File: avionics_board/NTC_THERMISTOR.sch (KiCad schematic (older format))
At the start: 2 parts

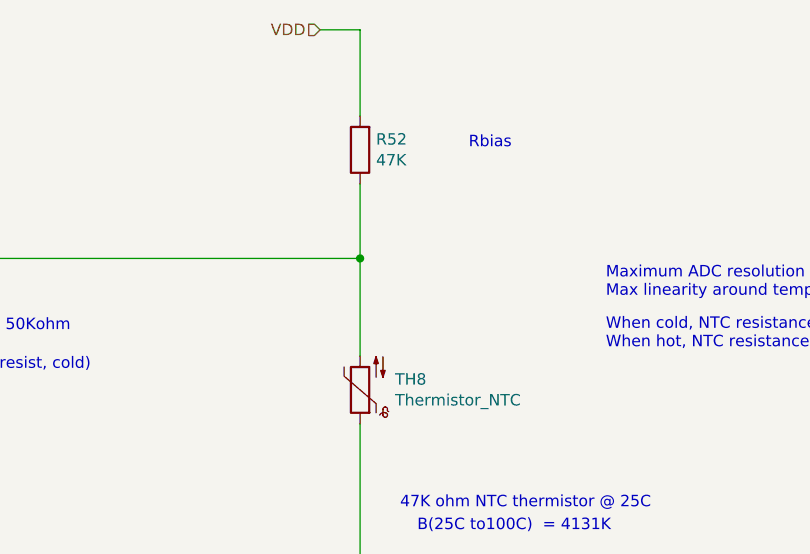
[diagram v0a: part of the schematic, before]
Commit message: Progress on EPS
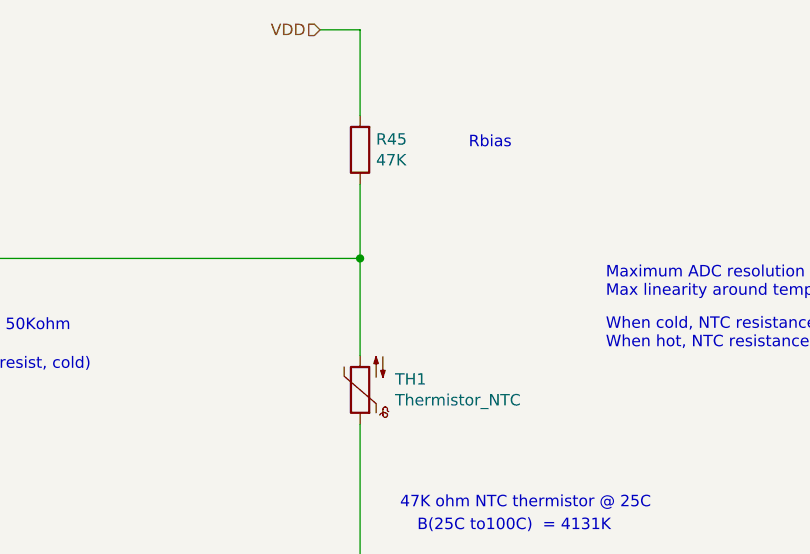
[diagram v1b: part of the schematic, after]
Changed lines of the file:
@@
 $Descr A 11000 8500
 encoding utf-8
-Sheet 14 25
+Sheet 13 24
 Title "NTC THERMISTOR"
 Date "2020-05-05"
@@
 AR Path="/5EA31C93/5EAB0B79/5EC02E3E/5EB42947" Ref="R51"  Part="1"
 AR Path="/5EA31C93/5EAB0B79/5EC02E43/5EB42947" Ref="R52"  Part="1"
-F 0 "R52" H 4680 1854 50  0000 R CNN
+F 0 "R45" H 4680 1854 50  0000 R CNN
 F 1 "47K" H 4680 1945 50  0000 R CNN
 F 2 "Resistor_SMD:R_0603_1608Metric_Pad1.05x0.95mm_HandSolder" V 4680 1900 50  0001 C CNN
@@
 AR Path="/5EA31C93/5EAB0B79/5EC02E3E/5EB41DDD" Ref="TH7"  Part="1"
 AR Path="/5EA31C93/5EAB0B79/5EC02E43/5EB41DDD" Ref="TH8"  Part="1"
-F 0 "TH8" H 4597 2904 50  0000 R CNN
+F 0 "TH1" H 4597 2904 50  0000 R CNN
 F 1 "Thermistor_NTC" H 4597 2995 50  0000 R CNN
 F 2 "Connector_PinHeader_1.27mm:PinHeader_1x02_P1.27mm_Vertical" H 4750 3000 50  0001 C CNN

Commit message: Essentially done with EPS schematic
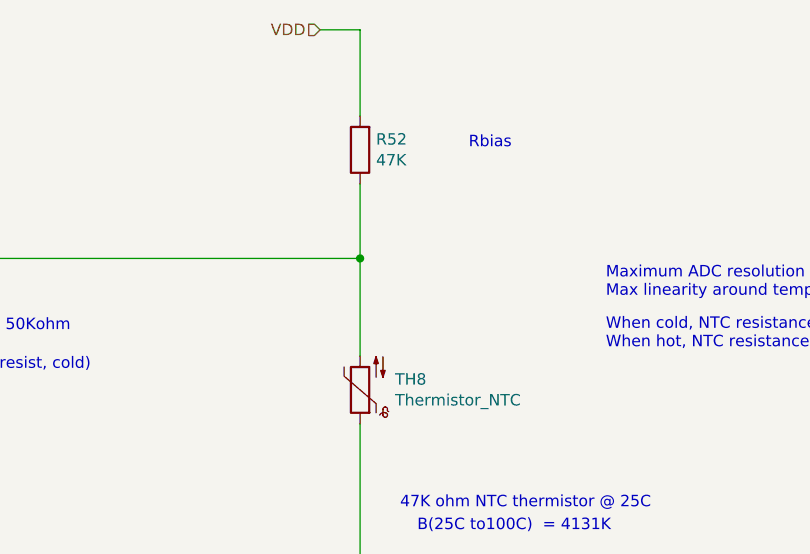
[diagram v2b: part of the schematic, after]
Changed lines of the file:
@@
 $Descr A 11000 8500
 encoding utf-8
-Sheet 13 24
+Sheet 13 23
 Title "NTC THERMISTOR"
 Date "2020-05-05"
@@
 AR Path="/5EA31C93/5EAB0B79/5EC02E3E/5EB42947" Ref="R51"  Part="1"
 AR Path="/5EA31C93/5EAB0B79/5EC02E43/5EB42947" Ref="R52"  Part="1"
-F 0 "R45" H 4680 1854 50  0000 R CNN
+F 0 "R52" H 4680 1854 50  0000 R CNN
 F 1 "47K" H 4680 1945 50  0000 R CNN
 F 2 "Resistor_SMD:R_0603_1608Metric_Pad1.05x0.95mm_HandSolder" V 4680 1900 50  0001 C CNN
@@
 AR Path="/5EA31C93/5EAB0B79/5EC02E3E/5EB41DDD" Ref="TH7"  Part="1"
 AR Path="/5EA31C93/5EAB0B79/5EC02E43/5EB41DDD" Ref="TH8"  Part="1"
-F 0 "TH1" H 4597 2904 50  0000 R CNN
+F 0 "TH8" H 4597 2904 50  0000 R CNN
 F 1 "Thermistor_NTC" H 4597 2995 50  0000 R CNN
 F 2 "Connector_PinHeader_1.27mm:PinHeader_1x02_P1.27mm_Vertical" H 4750 3000 50  0001 C CNN

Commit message: Update Avionics part names to match KiCad update. Update Avionics board to use new interboard connector
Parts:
- R45: footprint Resistor_SMD:R_0603_1608Metric_Pad1.05x0.95mm_HandSolder -> Resistor_SMD:R_0603_1608Metric_Pad0.98x0.95mm_HandSolder
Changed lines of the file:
@@
 F 0 "R52" H 4680 1854 50  0000 R CNN
 F 1 "47K" H 4680 1945 50  0000 R CNN
-F 2 "Resistor_SMD:R_0603_1608Metric_Pad1.05x0.95mm_HandSolder" V 4680 1900 50  0001 C CNN
+F 2 "Resistor_SMD:R_0603_1608Metric_Pad0.98x0.95mm_HandSolder" V 4680 1900 50  0001 C CNN
 F 3 "https://www.bourns.com/docs/Product-Datasheets/CHPREZTR.pdf" H 4750 1900 50  0001 C CNN
 F 4 "CR0603-FX-4702ELF" H 4750 1900 50  0001 C CNN "Mfr. #"
